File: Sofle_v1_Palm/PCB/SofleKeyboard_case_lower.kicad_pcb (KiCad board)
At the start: 2 copper layers, 137.2 x 109.2 mm, 0 parts

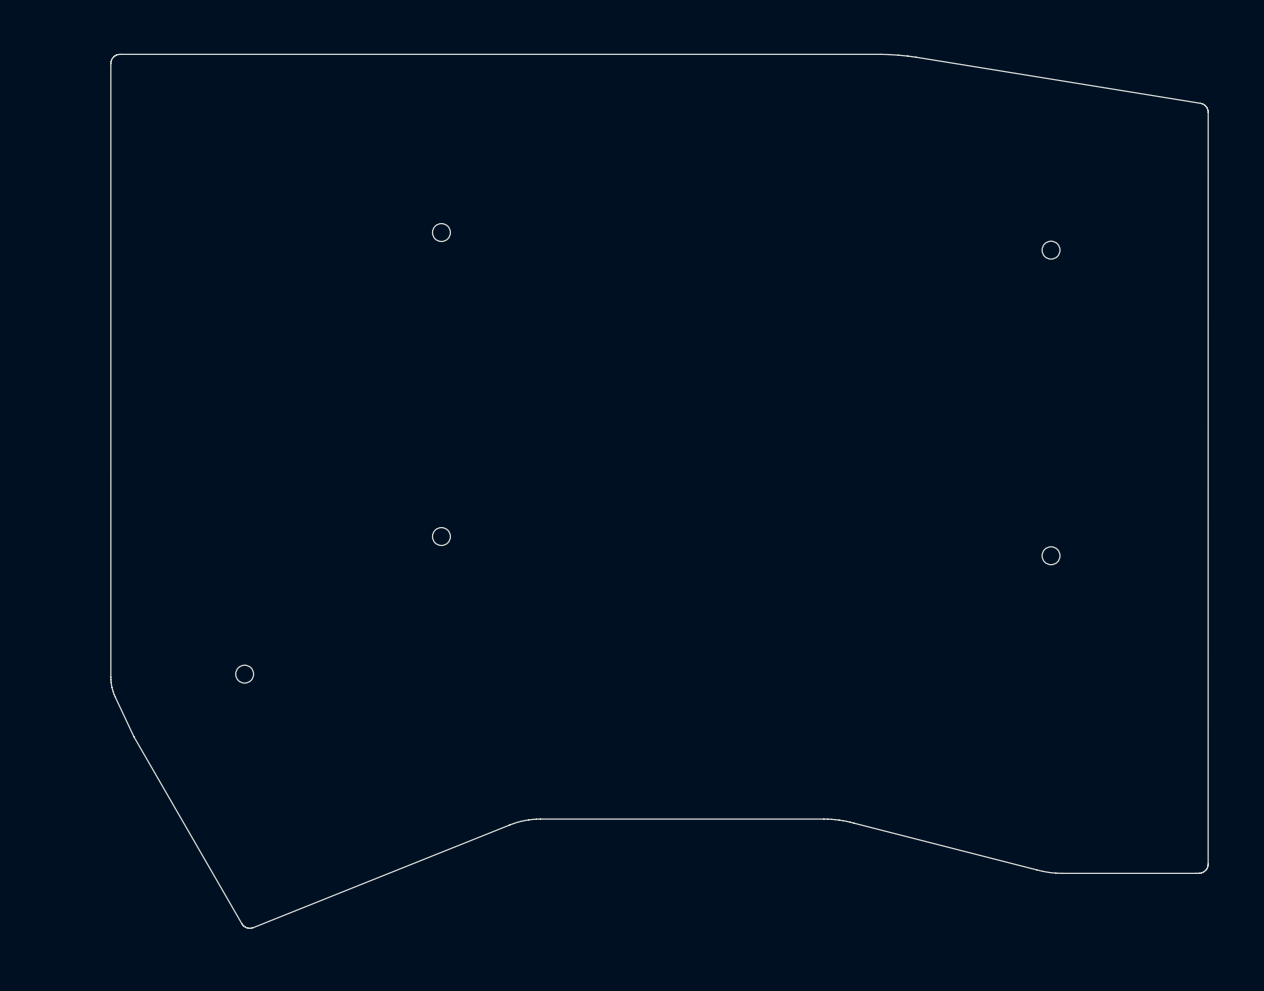
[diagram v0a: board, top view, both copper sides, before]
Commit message: Checkpoint commit.
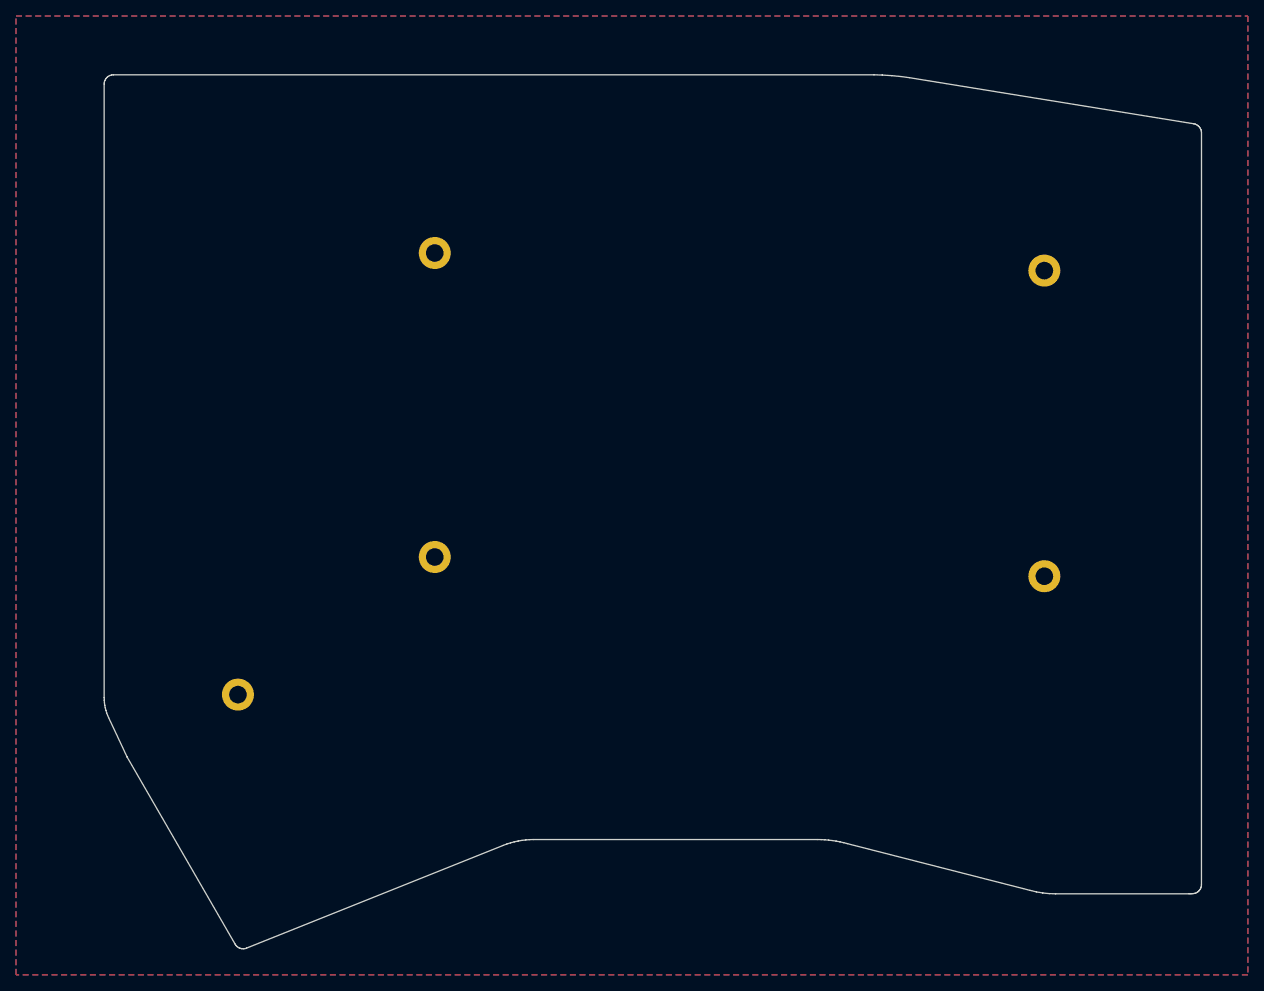
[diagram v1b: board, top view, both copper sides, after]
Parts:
- added ?: , , F.Cu at (205.0, 64.4)
- added ?: , , F.Cu at (104.2, 117.4)
- added ?: , , F.Cu at (128.8, 62.2)
- added ?: , , F.Cu at (205.0, 102.6)
- added ?: , , F.Cu at (128.8, 100.2)
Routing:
- added copper zone on B.Cu, net (none)
- added copper zone on F.Cu, net (none)
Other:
- outline, holes or cut-outs redrawn
